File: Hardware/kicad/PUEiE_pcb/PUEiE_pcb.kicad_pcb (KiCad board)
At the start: 2 copper layers, 52 x 96.1 mm, 121 parts, among them J101 Screw_Terminal_01x02, J102 USB_C_Receptacle_USB2.0_16P, J103 ST-LINKv2, J104 Conn_IPEX, J301 Conn_IPEX, J302 SMD_JST_PHx04, J303 JST_PHx04, J304 JST_PHx04, Q301 ZXMC4559DN8TA, SW101 SW_Push, SW201 SW_Nidec_CAS-120A1, U101 STM32WB55CGU6, U102 DLF162500LT-5028A1, U103 USBLC6-2SC6, U104 W25Q128JVSIQ, U201 TPS563240DDC, U202 AMS1117-3.3, U301 MAX-M10S-00B, U302 NC7WZ07P6X, U303 LIS3MDL, U304 TMC2208-LA, Y101 32MHz, Y102 32kHz768

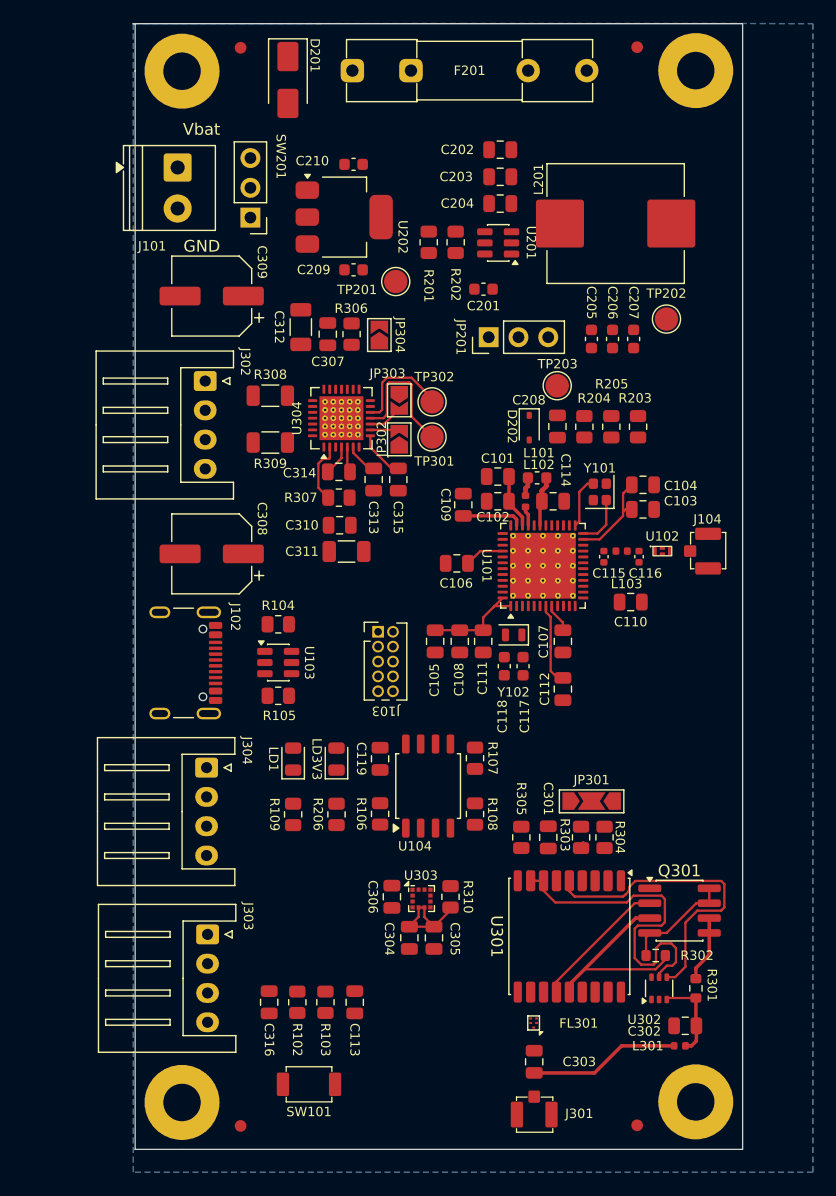
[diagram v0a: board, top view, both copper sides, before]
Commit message: Final PCB layout
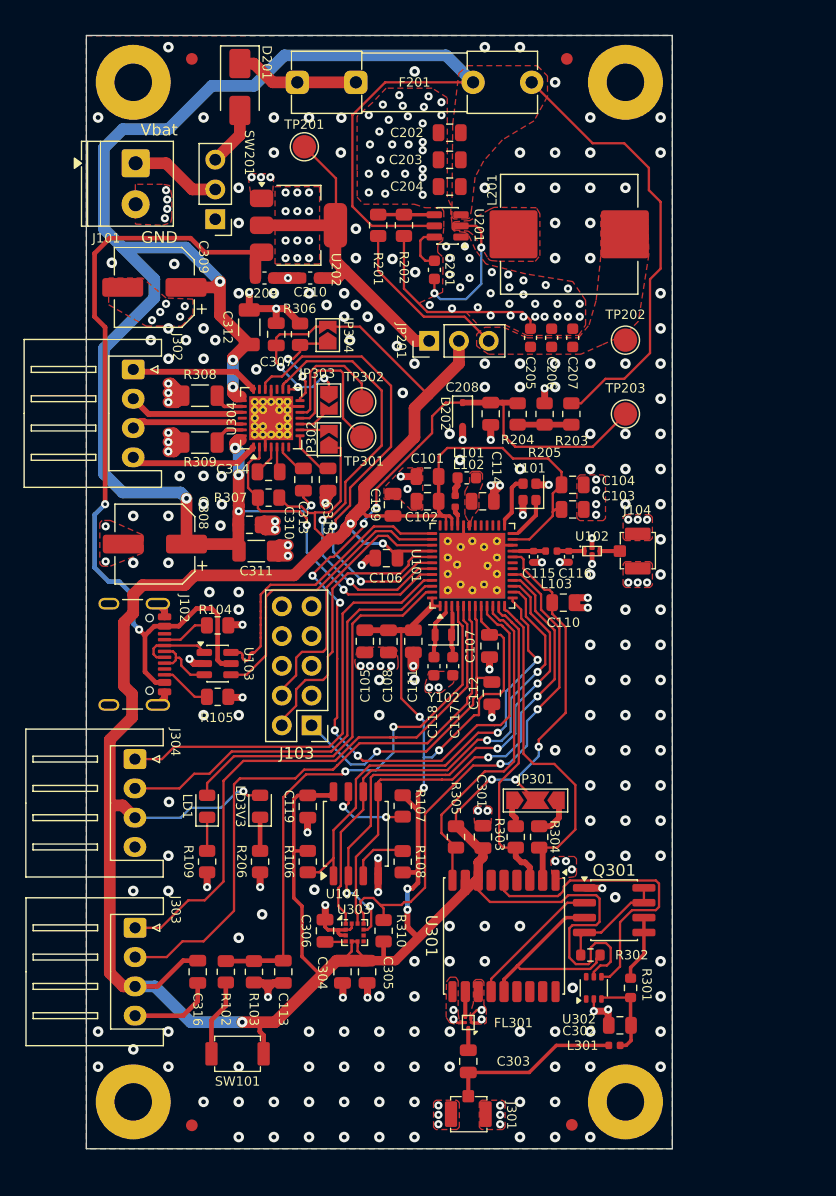
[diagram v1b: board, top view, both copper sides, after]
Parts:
- J103: footprint Connector_PinHeader_1.27mm:PinHeader_2x05_P1.27mm_Vertical -> Connector_PinHeader_2.54mm:PinHeader_2x05_P2.54mm_Vertical
- moved TP201 13.9 mm to (110.6, 86.5)
- moved C210 10.4 mm to (111.1, 97.7)
- moved J103 9.80 mm to (111.2, 135.9), turned to 180 degrees
- moved R109 8.37 mm to (102.3, 147.5)
- moved LD1 8.37 mm to (102.3, 142.8)
- moved C311 7.70 mm to (106.5, 121.0)
- moved C310 7.70 mm to (105.9, 118.8)
- moved R206 7.66 mm to (106.8, 147.5)
- moved LD3V3 7.66 mm to (106.8, 142.8)
- moved C209 7.63 mm to (107.2, 97.7)
- moved C119 7.39 mm to (110.9, 142.8)
- moved R106 7.39 mm to (110.9, 147.5)
- moved R107 7.39 mm to (119.0, 142.7)
- moved R108 7.39 mm to (119.0, 147.5), turned to -90 degrees
- moved U104 7.39 mm to (115.0, 145.1)
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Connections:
- J103 pad 10: SWCLK -> unconnected-(J103-Pin_10-Pad10)
- J103 pad 2: unconnected-(J103-Pin_2-Pad2) -> SWCLK
- J103 pad 3: GND -> unconnected-(J103-Pin_3-Pad3)
- J103 pad 4: unconnected-(J103-Pin_4-Pad4) -> SWDIO
- J103 pad 5: unconnected-(J103-Pin_5-Pad5) -> GND
- J103 pad 6: unconnected-(J103-Pin_6-Pad6) -> GND
- J103 pad 8: GND -> unconnected-(J103-Pin_8-Pad8)
- J103 pad 9: SWDIO -> unconnected-(J103-Pin_9-Pad9)
- U101 pad 14: /MAG_~{CS} -> /SPI_SCK
- U101 pad 15: /SPI_SCK -> /SPI_MISO
- U101 pad 16: /SPI_MISO -> /SPI_MOSI
- U101 pad 17: /SPI_MOSI -> /MAG_~{CS}
- U101 pad 36: /USER_LED_A -> unconnected-(U101-PA10-Pad36)
- U101 pad 42: /ADC_VBAT -> /SMD_DIR
- U101 pad 43: /MOTOR_PWM -> /SMD_STEP
- U101 pad 44: /MOTOR_DIR -> /SMD_ENN
- U101 pad 45: /SMD_DIR -> /MOTOR_DIR
- U101 pad 46: /SMD_STEP -> /MOTOR_PWM
- U101 pad 47: /SMD_ENN -> /USER_LED_A
- U101 pad 9: unconnected-(U101-PA0-Pad9) -> /ADC_VBAT
- U103 pad 4: /USB_D- -> /USB_D+
- U103 pad 6: /USB_D+ -> /USB_D-
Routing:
- net +3V3: track 70.8 -> 373.1 mm, vias 0 -> 15
- net +Vbat_fuse: track 0.00 -> 190.0 mm, vias 0 -> 8
- net GND: track 0.00 -> 113.8 mm, vias 0 -> 345
- net /ADC_VBAT: track 0.00 -> 82.9 mm, vias 0 -> 6
- net VUSB: track 0.00 -> 70.3 mm, vias 0 -> 2
- net /I2C_SDA: track 0.00 -> 52.2 mm
- net /I2C_SCL: track 0.00 -> 48.9 mm
- net /BOOT0: track 0.00 -> 46.3 mm, vias 0 -> 2
- net /SPI_MISO: track 0.00 -> 45.1 mm, vias 0 -> 4
- net /MAG_~{CS}: track 0.00 -> 45.1 mm, vias 0 -> 2
- net /SPI_MOSI: track 0.00 -> 43.4 mm, vias 0 -> 2
- net /SPI_SCK: track 0.00 -> 42.5 mm, vias 0 -> 2
- net /MEM_~{CS}: track 0.00 -> 39.3 mm, vias 0 -> 2
- net /SMD_DIR: track 0.00 -> 39.2 mm, vias 0 -> 2
- net /SMD_STEP: track 0.00 -> 38.2 mm, vias 0 -> 2
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- added copper zone on F.Cu, net +3V3
- added copper zone on F.Cu, net +Vbat_fuse
- added copper zone on F.Cu, net /+3.3V Regulator/+3.3Vbat
- added copper zone on F.Cu, net /+3.3V Regulator/LDO_SW
- added copper zone on F.Cu, net /VFBSMPS
- added copper zone on F.Cu, net GND
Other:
- board size 52 x 96.1 mm -> 50 x 95 mm
